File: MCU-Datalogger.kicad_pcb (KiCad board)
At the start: 2 copper layers, 51.1 x 30 mm, 29 parts, among them J1 Conn_01x04_Pin, J2 Conn_01x04_Pin, J3 Conn_01x09_Pin, J4 Conn_02x03_Odd_Even, U1 24LC1025, U2 24LC1025, U3 DS1337S_, U4 ATMEGA328P-AU, Y1 32.768 KHz, Y2 16 MHz

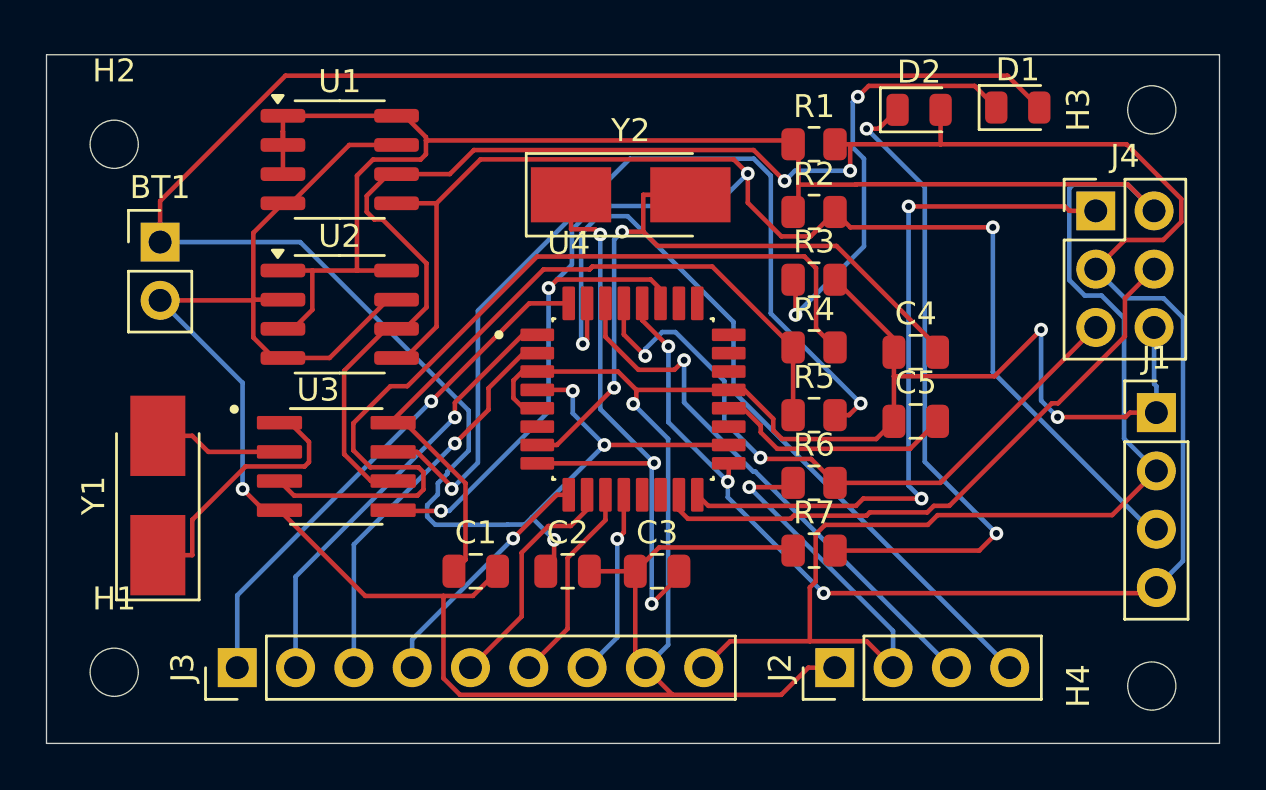
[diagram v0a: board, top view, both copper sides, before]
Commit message: fix bugs
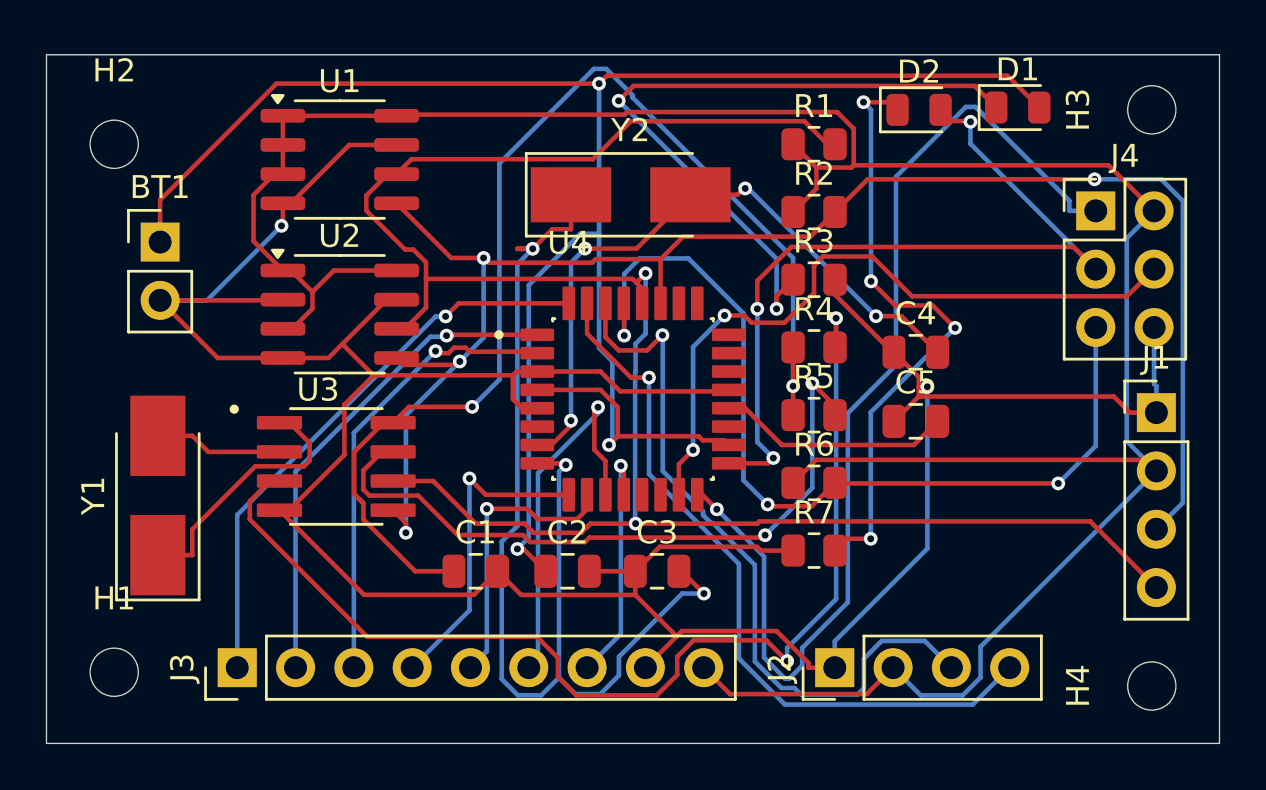
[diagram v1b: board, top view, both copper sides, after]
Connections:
- D2 pad 2: /SCL -> /SCK
- J4 pad 3: /SCL -> /SCK
- U4 pad 17: /SCL -> /SCK
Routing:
- net /SCK: track 0.00 -> 36.0 mm, vias 0 -> 3
- net /SCL: track 112.3 -> 87.7 mm, vias 5 -> 2
- net Net-(U4-PB7): track 27.0 -> 49.7 mm
- net Net-(U3-VCC): track 33.2 -> 51.8 mm, vias 0 -> 2
- net /MISO: track 31.3 -> 45.8 mm, vias 2 -> 1
- net /SDA: track 85.0 -> 71.5 mm
- net Net-(D1-K): track 19.2 -> 30.6 mm
- net /RESET: track 29.5 -> 39.9 mm, vias 2 -> 3
- net Net-(U3-SQW/~INT): track 40.2 -> 30.3 mm
- net Net-(U3-~{INTA}): track 39.2 -> 48.5 mm, vias 0 -> 2
- net GND: track 145.9 -> 136.7 mm, vias 4 -> 2
- net /RX: track 23.9 -> 31.8 mm
- net /D7: track 8.91 -> 16.7 mm, vias 0 -> 1
- net /VCC: track 122.4 -> 117.1 mm, vias 1 -> 0
- net /TX: track 35.6 -> 32.0 mm
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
